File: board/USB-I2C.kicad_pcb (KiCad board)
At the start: 2 copper layers, 44 x 18 mm, 17 parts, among them J1 USB_OTG, J2 Conn_01x06, U1 SPX3819, U2 ATSAMD11C14A-SS, X1 I2C-6P, X2 I2C, X3 SWD

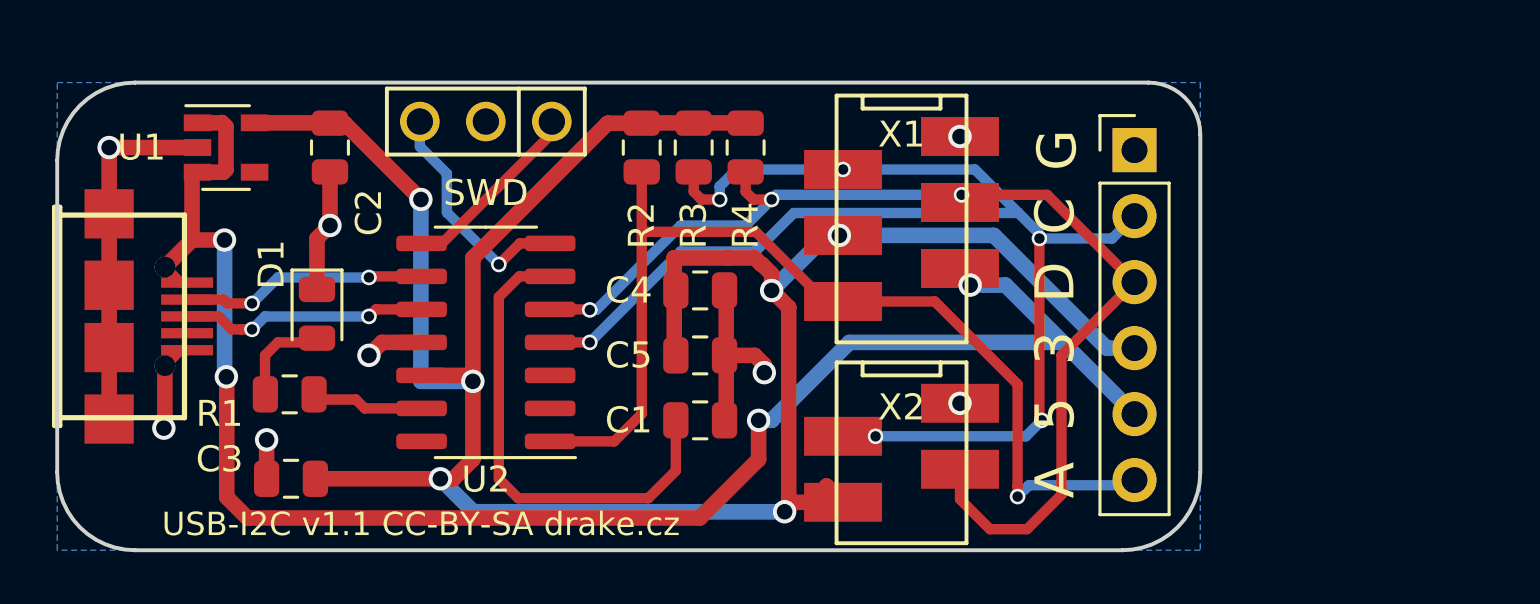
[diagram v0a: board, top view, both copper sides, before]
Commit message: WIP
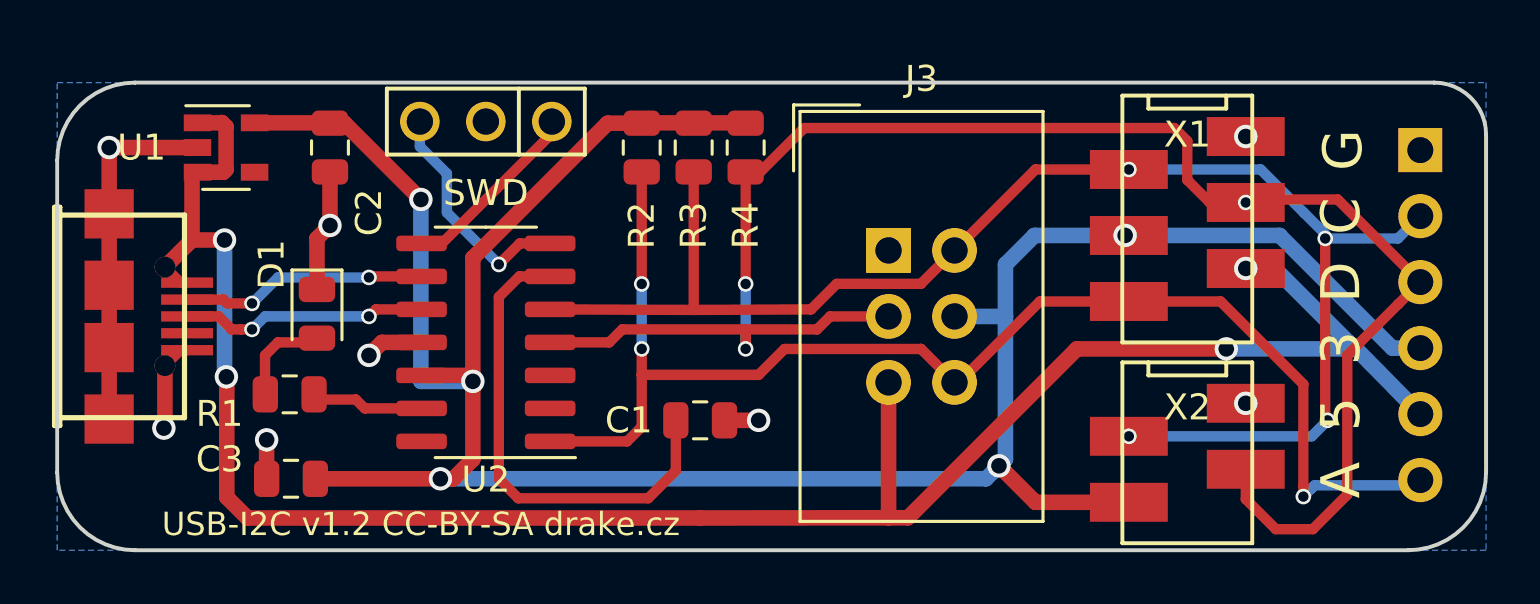
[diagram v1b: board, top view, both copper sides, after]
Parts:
- removed C4, C5: 100n, Capacitor_SMD:C_0805_2012Metric
- added J3: Conn_01x06, Connector_IDC:IDC-Header_2x03_P2.54mm_Vertical, F.Cu at (179.0, 105.5)
- J2: moved to B.Cu
- moved J2 11.0 mm to (199.5, 101.6), turned to 180 degrees
- moved X1 11.0 mm to (190.5, 104.2)
- moved X2 11.0 mm to (190.5, 113.2)
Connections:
- J1 pad 4: Net-(J1-Pad4) -> (no net)
- U1 pad 4: Net-(U1-Pad4) -> (no net)
- U2 pad 14: Net-(U2-Pad14) -> (no net)
- U2 pad 2: Net-(U2-Pad2) -> (no net)
- U2 pad 3: Net-(U2-Pad3) -> (no net)
- U2 pad 4: /SCL -> /SDA
- U2 pad 5: /SDA -> /SCL
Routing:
- net /SDA: track 43.0 -> 66.5 mm
- net +5V: track 65.3 -> 81.5 mm
- net /ALERT: track 39.3 -> 52.4 mm, vias 1 -> 3
- net GND: track 32.3 -> 26.7 mm
- net +3V3: track 96.4 -> 100.8 mm, vias 6 -> 5
- net /SCL: track 54.0 -> 57.5 mm, vias 6 -> 4
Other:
- board size 44 x 18 mm -> 55 x 18 mm
- board text added: "USB-I2C v1.2 CC-BY-SA drake.cz"
- board text removed: "USB-I2C v1.1 CC-BY-SA drake.cz"
